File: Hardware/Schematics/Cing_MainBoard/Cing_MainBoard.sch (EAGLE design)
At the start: 141 parts, among them IC1 L293D, IC2 LM2576S, IC3 FT232RL, IC5 BME280, Q1 16mhz, Q2 BSS138, Q3 BSS138, Q4 BSS138, Q5 BSS138, Q7 NP2301AMR-G, U3 MPU-6050MPU6050

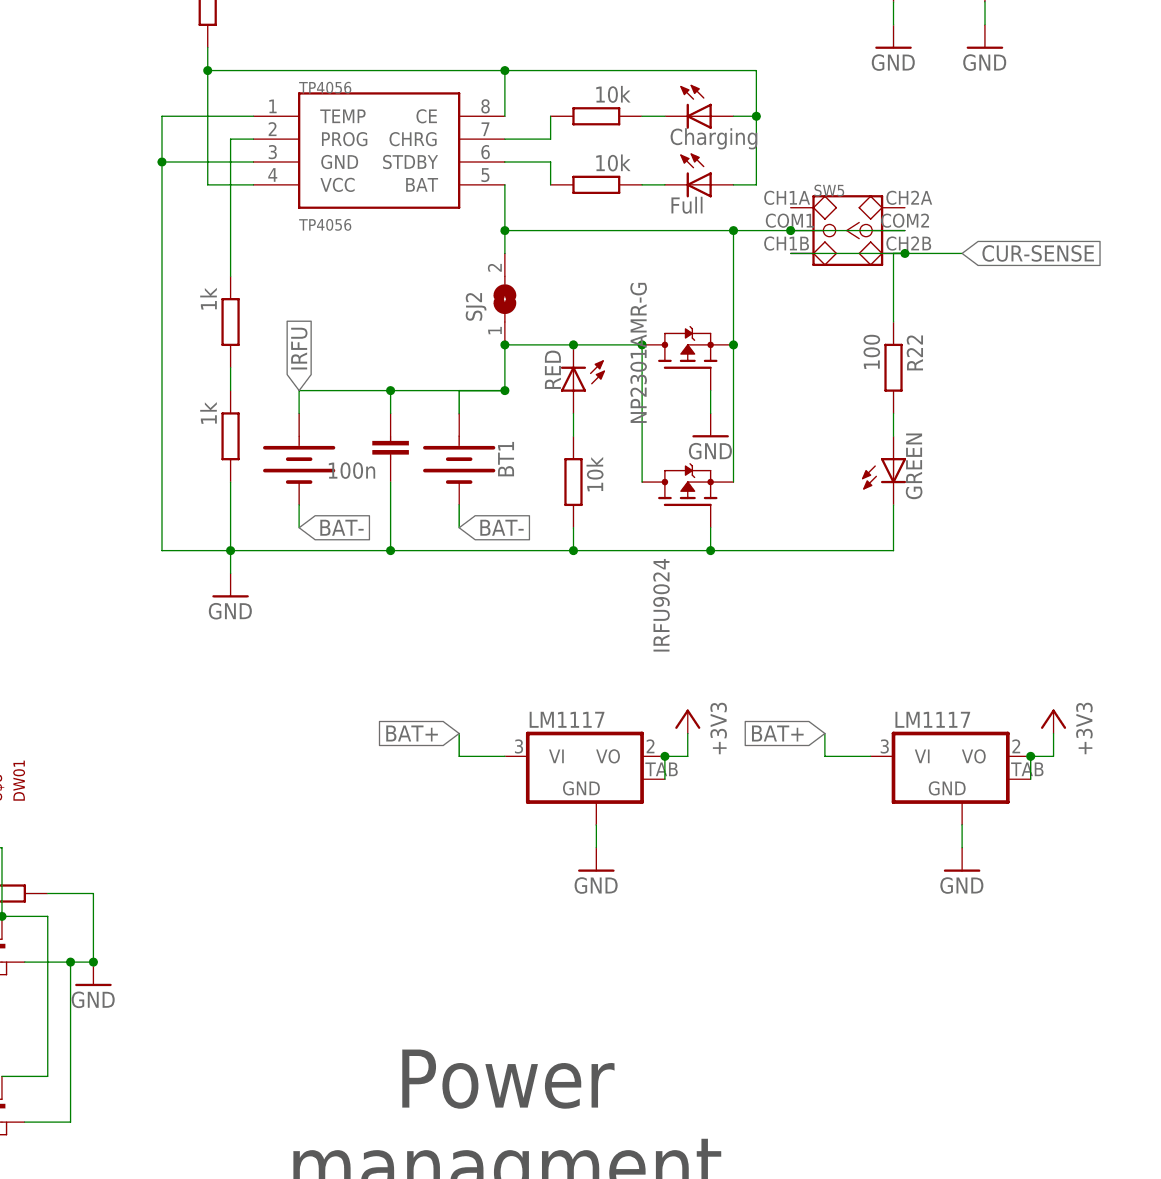
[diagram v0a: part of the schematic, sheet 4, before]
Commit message: commit
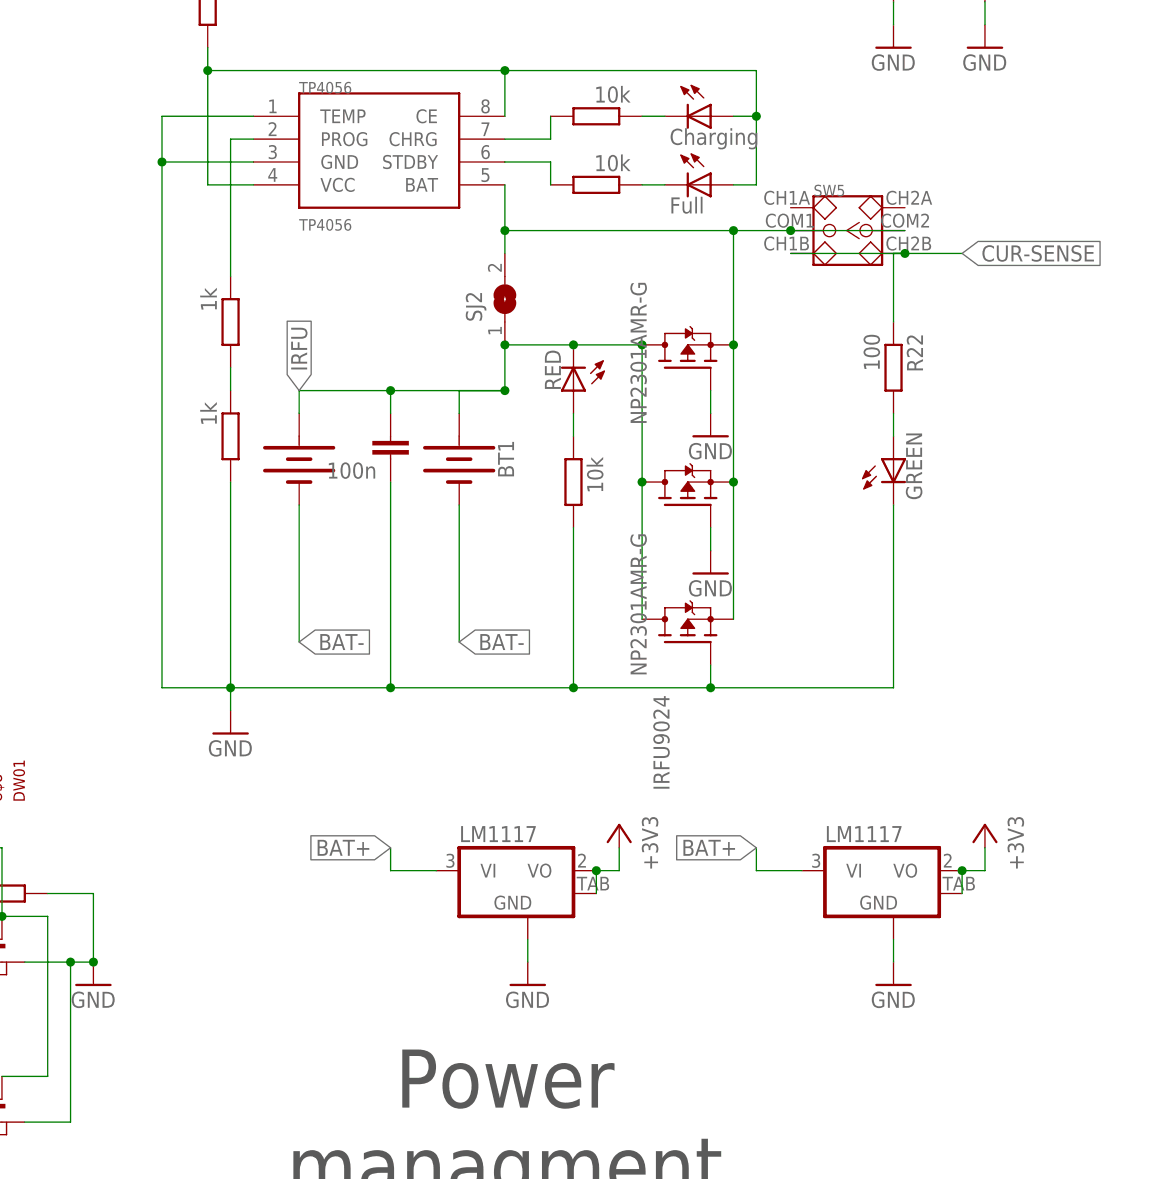
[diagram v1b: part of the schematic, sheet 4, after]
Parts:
- added Q6: NP2301AMR-G, transistor-fet:BSA223SP
- added U$15: (no value), diy-modules:COMPASS-HMC5883L
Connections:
- net +3V3: now also U$15.VCC
- net GND: now also Q6.G, U$15.GND
- net IRFU: now also Q6.D
- net N$26: now also Q6.S
- net SCL: now also U$15.SCL
- net SDA: now also U$15.SDA

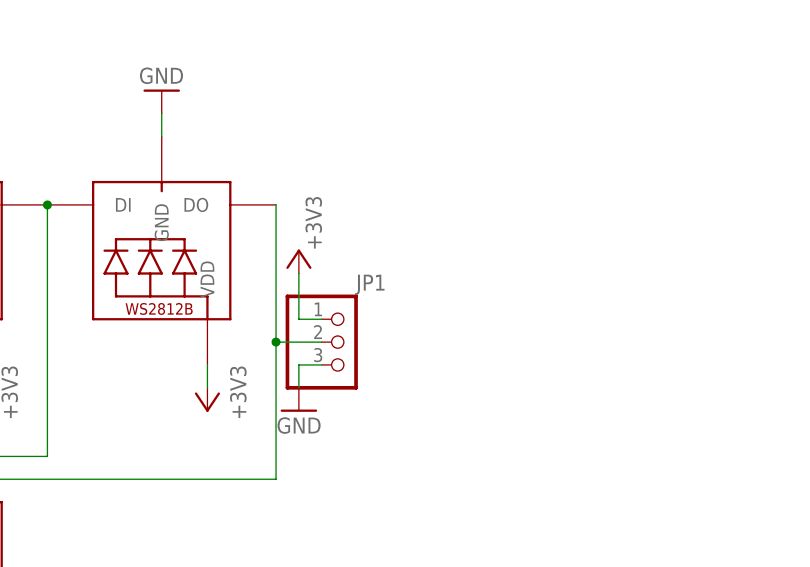
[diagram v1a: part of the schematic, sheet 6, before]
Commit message: commit
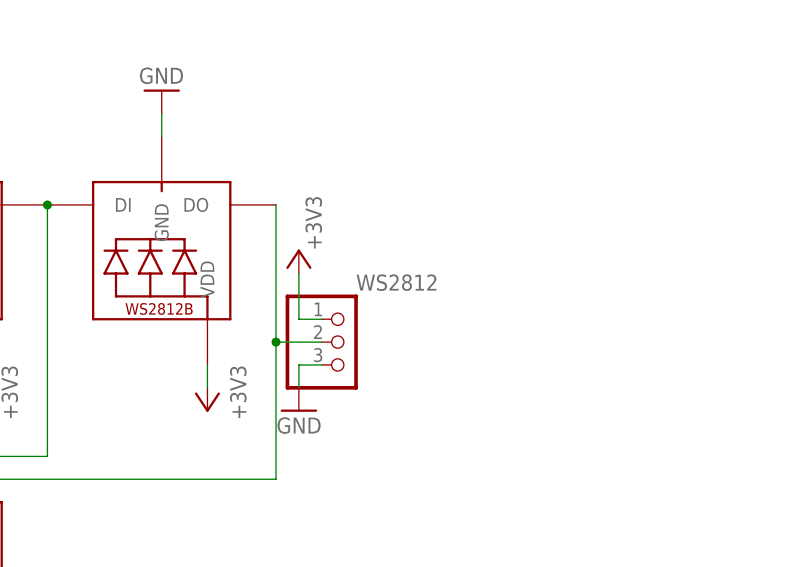
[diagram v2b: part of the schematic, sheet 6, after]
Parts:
- renumbered JP1 to WS2812
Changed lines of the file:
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@@
 <part name="GND52" library="supply1" library_urn="urn:adsk.eagle:library:371" deviceset="GND" device=""/>
 <part name="GND53" library="supply1" library_urn="urn:adsk.eagle:library:371" deviceset="GND" device=""/>
-<part name="JP1" library="pinhead" library_urn="urn:adsk.eagle:library:325" deviceset="PINHD-1X3" device="" package3d_urn="urn:adsk.eagle:package:22458/2"/>
+<part name="WS2812" library="pinhead" library_urn="urn:adsk.eagle:library:325" deviceset="PINHD-1X3" device="" package3d_urn="urn:adsk.eagle:package:22458/2"/>
 <part name="GND54" library="supply1" library_urn="urn:adsk.eagle:library:371" deviceset="GND" device=""/>
 <part name="+3V27" library="supply1" library_urn="urn:adsk.eagle:library:371" deviceset="+3V3" device=""/>
@@
 <attribute name="VALUE" x="43.18" y="96.52" size="1.778" layer="96" rot="MR180"/>
 </instance>
-<instance part="JP1" gate="A" x="142.24" y="66.04" smashed="yes">
+<instance part="WS2812" gate="A" x="142.24" y="66.04" smashed="yes">
 <attribute name="NAME" x="143.51" y="71.755" size="1.778" layer="95"/>
 <attribute name="VALUE" x="135.89" y="58.42" size="1.778" layer="96"/>
@@
 </segment>
 <segment>
-<pinref part="JP1" gate="A" pin="3"/>
+<pinref part="WS2812" gate="A" pin="3"/>
 <wire x1="139.7" y1="63.5" x2="137.16" y2="63.5" width="0.1524" layer="91"/>
 <pinref part="GND54" gate="1" pin="GND"/>
@@
 </segment>
 <segment>
-<pinref part="JP1" gate="A" pin="1"/>
+<pinref part="WS2812" gate="A" pin="1"/>
 <wire x1="139.7" y1="68.58" x2="137.16" y2="68.58" width="0.1524" layer="91"/>
 <pinref part="+3V27" gate="G$1" pin="+3V3"/>
@@
 <wire x1="134.62" y1="66.04" x2="139.7" y2="66.04" width="0.1524" layer="91"/>
 <junction x="134.62" y="66.04"/>
-<pinref part="JP1" gate="A" pin="2"/>
+<pinref part="WS2812" gate="A" pin="2"/>
 </segment>
 </net>
